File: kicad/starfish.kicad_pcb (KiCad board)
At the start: 2 copper layers, 50 x 38.4 mm, 6 parts, among them J1 Conn_01x09, J2 conn1, J3 Conn_01x08, J4 Conn_01x08, J5 conn2, J6 Conn_01x05

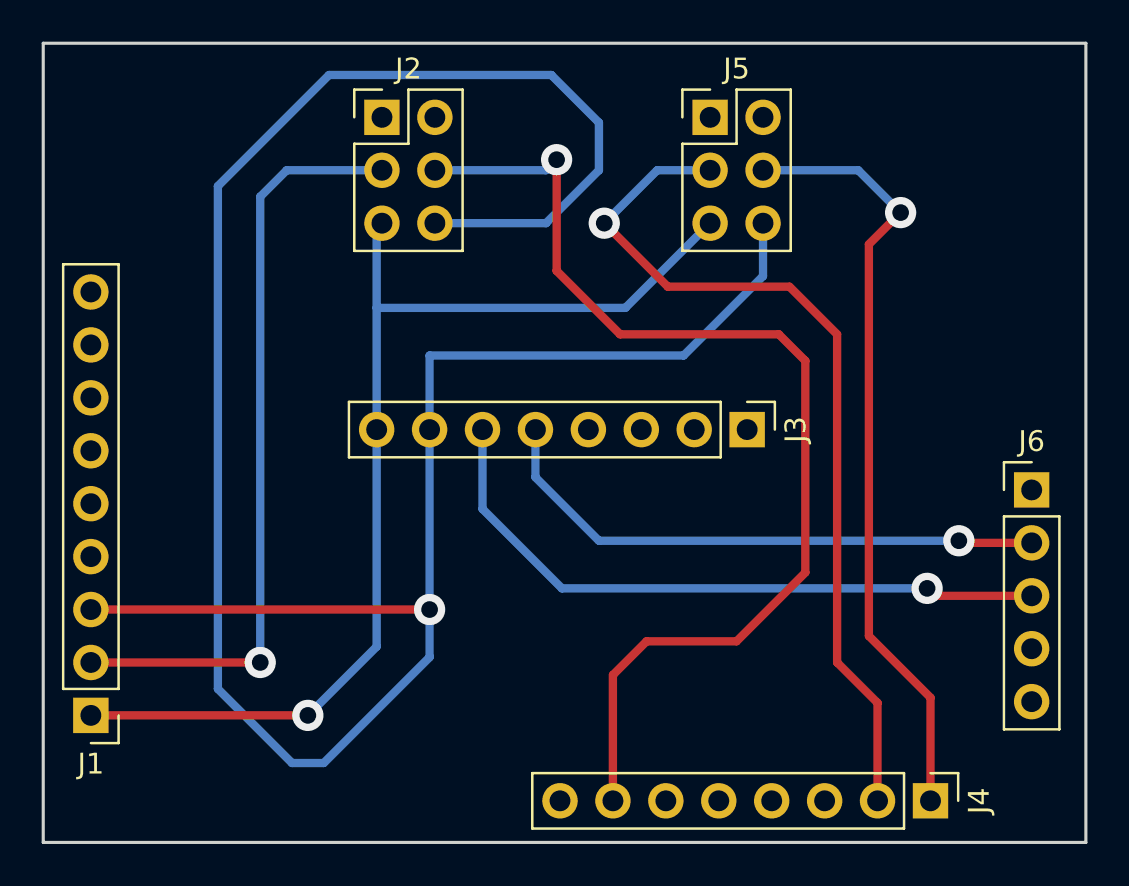
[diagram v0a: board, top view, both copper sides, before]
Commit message: shield
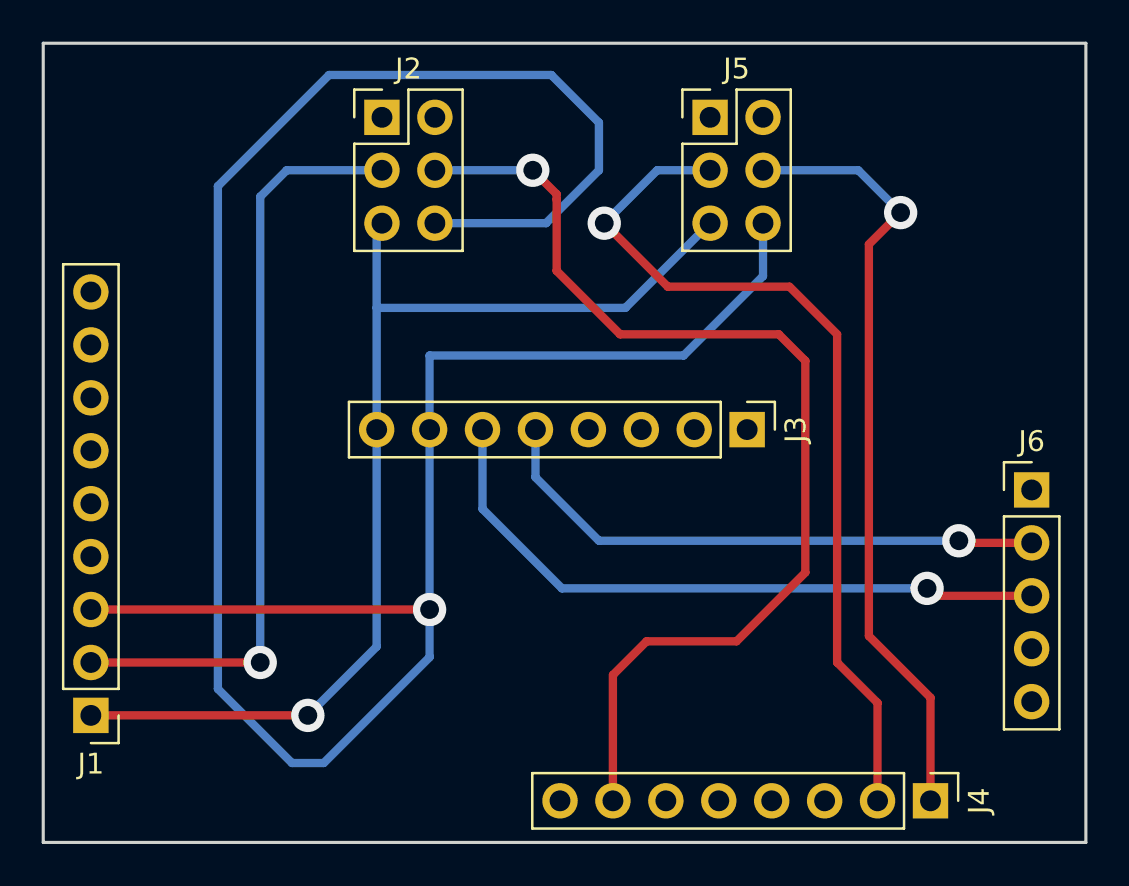
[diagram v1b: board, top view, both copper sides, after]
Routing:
- net Net-(J2-Pad2): track 52.6 -> 51.2 mm
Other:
- net class Default: via_dia 1.5 -> 1.6; via_drill 0.8 -> 0.9
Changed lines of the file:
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@@
     (links 13)
     (no_connects 1)
-    (area 116.510999 104.826999 166.699001 143.331001)
+    (area 116.246999 104.553 166.699001 143.884561)
     (thickness 1.6)
     (drawings 4)
-    (tracks 72)
+    (tracks 74)
     (zones 0)
     (modules 6)
@@
     (segment_width 0.2)
     (edge_width 0.15)
-    (via_size 1.5)
-    (via_drill 0.8)
+    (via_size 1.6)
+    (via_drill 0.9)
     (via_min_size 0.4)
     (via_min_drill 0.3)
@@
     (visible_elements 7FFFFFFF)
     (pcbplotparams
-      (layerselection 0x00000_80000001)
+      (layerselection 0x01000_80000001)
       (usegerberextensions false)
       (excludeedgelayer true)
@@
     (clearance 0.8)
     (trace_width 0.4)
-    (via_dia 1.5)
-    (via_drill 0.8)
+    (via_dia 1.6)
+    (via_drill 0.9)
     (uvia_dia 0.3)
     (uvia_drill 0.1)
@@
   (gr_line (start 166.624 143.256) (end 116.586 143.256) (angle 90) (layer Edge.Cuts) (width 0.15))
   (segment (start 132.588 117.602) (end 144.526 117.602) (width 0.4) (layer B.Cu) (net 1))
-  (segment (start 144.526 117.602) (end 148.59 113.538) (width 0.4) (layer B.Cu) (net 1) (status 800000))
+  (segment (start 144.526 117.602) (end 148.59 113.538) (width 0.4) (layer B.Cu) (net 1))
   (segment (start 132.588 123.444) (end 132.588 117.602) (width 0.4) (layer B.Cu) (net 1))
   (segment (start 132.588 117.602) (end 132.588 113.792) (width 0.4) (layer B.Cu) (net 1))
@@
   (segment (start 132.588 133.858) (end 132.588 123.444) (width 0.4) (layer B.Cu) (net 1))
   (segment (start 129.286 137.16) (end 132.588 133.858) (width 0.4) (layer B.Cu) (net 1))
-  (via (at 129.286 137.16) (size 1.5) (drill 0.8) (layers F.Cu B.Cu) (net 1))
-  (segment (start 132.842 110.998) (end 128.27 110.998) (width 0.4) (layer B.Cu) (net 2) (status 400000))
-  (segment (start 127 134.62) (end 118.872 134.62) (width 0.4) (layer F.Cu) (net 2) (status 800000))
-  (via (at 127 134.62) (size 1.5) (drill 0.8) (layers F.Cu B.Cu) (net 2))
+  (via (at 129.286 137.16) (size 1.6) (drill 0.9) (layers F.Cu B.Cu) (net 1))
+  (segment (start 132.842 110.998) (end 128.27 110.998) (width 0.4) (layer B.Cu) (net 2))
+  (segment (start 127 134.62) (end 118.872 134.62) (width 0.4) (layer F.Cu) (net 2))
+  (via (at 127 134.62) (size 1.6) (drill 0.9) (layers F.Cu B.Cu) (net 2))
   (segment (start 127 112.268) (end 127 134.62) (width 0.4) (layer B.Cu) (net 2))
   (segment (start 128.27 110.998) (end 127 112.268) (width 0.4) (layer B.Cu) (net 2))
   (segment (start 135.128 132.08) (end 135.128 134.366) (width 0.4) (layer B.Cu) (net 3))
-  (segment (start 140.716 113.538) (end 135.382 113.538) (width 0.4) (layer B.Cu) (net 3) (status 800000))
+  (segment (start 140.716 113.538) (end 135.382 113.538) (width 0.4) (layer B.Cu) (net 3))
   (segment (start 143.256 110.998) (end 140.716 113.538) (width 0.4) (layer B.Cu) (net 3))
   (segment (start 143.256 108.712) (end 143.256 110.998) (width 0.4) (layer B.Cu) (net 3))
@@
   (segment (start 130.048 139.446) (end 128.524 139.446) (width 0.4) (layer B.Cu) (net 3))
   (segment (start 135.128 134.366) (end 130.048 139.446) (width 0.4) (layer B.Cu) (net 3))
-  (segment (start 151.13 113.538) (end 151.13 116.078) (width 0.4) (layer B.Cu) (net 3) (status 400000))
+  (segment (start 151.13 113.538) (end 151.13 116.078) (width 0.4) (layer B.Cu) (net 3))
   (segment (start 147.32 119.888) (end 135.128 119.888) (width 0.4) (layer B.Cu) (net 3))
   (segment (start 151.13 116.078) (end 147.32 119.888) (width 0.4) (layer B.Cu) (net 3))
@@
   (segment (start 118.872 132.08) (end 135.128 132.08) (width 0.4) (layer F.Cu) (net 3))
   (segment (start 135.128 132.08) (end 135.128 123.444) (width 0.4) (layer B.Cu) (net 3))
-  (via (at 135.128 132.08) (size 1.5) (drill 0.8) (layers F.Cu B.Cu) (net 3))
-  (segment (start 164.02304 128.8796) (end 160.6296 128.8796) (width 0.4) (layer F.Cu) (net 16) (status 400000))
-  (segment (start 140.208 125.73) (end 140.208 123.444) (width 0.4) (layer B.Cu) (net 16) (status 800000))
+  (via (at 135.128 132.08) (size 1.6) (drill 0.9) (layers F.Cu B.Cu) (net 3))
+  (segment (start 164.02304 128.8796) (end 160.6296 128.8796) (width 0.4) (layer F.Cu) (net 16))
+  (segment (start 140.208 125.73) (end 140.208 123.444) (width 0.4) (layer B.Cu) (net 16))
   (segment (start 143.256 128.778) (end 140.208 125.73) (width 0.4) (layer B.Cu) (net 16))
   (segment (start 160.528 128.778) (end 143.256 128.778) (width 0.4) (layer B.Cu) (net 16))
-  (via (at 160.528 128.778) (size 1.5) (drill 0.8) (layers F.Cu B.Cu) (net 16))
+  (via (at 160.528 128.778) (size 1.6) (drill 0.9) (layers F.Cu B.Cu) (net 16))
   (segment (start 160.6296 128.8796) (end 160.528 128.778) (width 0.4) (layer F.Cu) (net 16))
-  (segment (start 164.02304 131.4196) (end 159.3596 131.4196) (width 0.4) (layer F.Cu) (net 17) (status 400000))
-  (segment (start 137.668 127.254) (end 137.668 123.444) (width 0.4) (layer B.Cu) (net 17) (status 800000))
+  (segment (start 164.02304 131.4196) (end 159.3596 131.4196) (width 0.4) (layer F.Cu) (net 17))
+  (segment (start 137.668 127.254) (end 137.668 123.444) (width 0.4) (layer B.Cu) (net 17))
   (segment (start 141.478 131.064) (end 137.668 127.254) (width 0.4) (layer B.Cu) (net 17))
   (segment (start 159.004 131.064) (end 141.478 131.064) (width 0.4) (layer B.Cu) (net 17))
-  (via (at 159.004 131.064) (size 1.5) (drill 0.8) (layers F.Cu B.Cu) (net 17))
+  (via (at 159.004 131.064) (size 1.6) (drill 0.9) (layers F.Cu B.Cu) (net 17))
   (segment (start 159.3596 131.4196) (end 159.004 131.064) (width 0.4) (layer F.Cu) (net 17))
-  (segment (start 148.59 110.998) (end 146.05 110.998) (width 0.4) (layer B.Cu) (net 18) (status 400000))
-  (segment (start 156.62656 136.56056) (end 156.62656 141.25956) (width 0.4) (layer F.Cu) (net 18) (status 800000))
+  (segment (start 148.59 110.998) (end 146.05 110.998) (width 0.4) (layer B.Cu) (net 18))
+  (segment (start 156.62656 136.56056) (end 156.62656 141.25956) (width 0.4) (layer F.Cu) (net 18))
   (segment (start 154.686 134.62) (end 156.62656 136.56056) (width 0.4) (layer F.Cu) (net 18))
   (segment (start 154.686 118.872) (end 154.686 134.62) (width 0.4) (layer F.Cu) (net 18))
@@
   (segment (start 146.558 116.586) (end 152.4 116.586) (width 0.4) (layer F.Cu) (net 18))
   (segment (start 143.51 113.538) (end 146.558 116.586) (width 0.4) (layer F.Cu) (net 18))
-  (via (at 143.51 113.538) (size 1.5) (drill 0.8) (layers F.Cu B.Cu) (net 18))
+  (via (at 143.51 113.538) (size 1.6) (drill 0.9) (layers F.Cu B.Cu) (net 18))
   (segment (start 146.05 110.998) (end 143.51 113.538) (width 0.4) (layer B.Cu) (net 18))
-  (segment (start 135.382 110.998) (end 140.716 110.998) (width 0.4) (layer B.Cu) (net 27) (status 400000))
-  (segment (start 143.92656 135.21944) (end 143.92656 141.25956) (width 0.4) (layer F.Cu) (net 27) (status 800000))
+  (segment (start 139.7 110.998) (end 140.081 110.998) (width 0.4) (layer B.Cu) (net 27))
+  (segment (start 141.224 112.395) (end 141.224 115.824) (width 0.4) (layer F.Cu) (net 27))
+  (segment (start 141.224 115.824) (end 144.272 118.872) (width 0.4) (layer F.Cu) (net 27))
+  (segment (start 144.272 118.872) (end 151.892 118.872) (width 0.4) (layer F.Cu) (net 27))
+  (segment (start 151.892 118.872) (end 153.162 120.142) (width 0.4) (layer F.Cu) (net 27))
+  (segment (start 153.162 120.142) (end 153.162 130.302) (width 0.4) (layer F.Cu) (net 27))
+  (segment (start 153.162 130.302) (end 149.86 133.604) (width 0.4) (layer F.Cu) (net 27))
+  (segment (start 149.86 133.604) (end 145.542 133.604) (width 0.4) (layer F.Cu) (net 27))
   (segment (start 145.542 133.604) (end 143.92656 135.21944) (width 0.4) (layer F.Cu) (net 27))
-  (segment (start 149.86 133.604) (end 145.542 133.604) (width 0.4) (layer F.Cu) (net 27))
-  (segment (start 153.162 130.302) (end 149.86 133.604) (width 0.4) (layer F.Cu) (net 27))
-  (segment (start 153.162 120.142) (end 153.162 130.302) (width 0.4) (layer F.Cu) (net 27))
-  (segment (start 151.892 118.872) (end 153.162 120.142) (width 0.4) (layer F.Cu) (net 27))
-  (segment (start 144.272 118.872) (end 151.892 118.872) (width 0.4) (layer F.Cu) (net 27))
-  (segment (start 141.224 115.824) (end 144.272 118.872) (width 0.4) (layer F.Cu) (net 27))
-  (segment (start 141.224 110.49) (end 141.224 115.824) (width 0.4) (layer F.Cu) (net 27))
-  (via (at 141.224 110.49) (size 1.5) (drill 0.8) (layers F.Cu B.Cu) (net 27))
-  (segment (start 140.716 110.998) (end 141.224 110.49) (width 0.4) (layer B.Cu) (net 27))
-  (segment (start 151.13 110.998) (end 155.702 110.998) (width 0.4) (layer B.Cu) (net 28) (status 400000))
-  (segment (start 159.16656 136.30656) (end 159.16656 141.25956) (width 0.4) (layer F.Cu) (net 28) (status 800000))
+  (segment (start 143.92656 141.25956) (end 143.92656 135.21944) (width 0.4) (layer F.Cu) (net 27))
+  (segment (start 139.7 110.998) (end 135.382 110.998) (width 0.4) (layer B.Cu) (net 27) (status 800000))
+  (segment (start 141.224 112.141) (end 141.224 112.395) (width 0.4) (layer F.Cu) (net 27))
+  (segment (start 140.081 110.998) (end 141.224 112.141) (width 0.4) (layer F.Cu) (net 27))
+  (via (at 140.081 110.998) (size 1.6) (drill 0.9) (layers F.Cu B.Cu) (net 27))
+  (segment (start 151.13 110.998) (end 155.702 110.998) (width 0.4) (layer B.Cu) (net 28))
+  (segment (start 159.16656 136.30656) (end 159.16656 141.25956) (width 0.4) (layer F.Cu) (net 28))
   (segment (start 156.21 133.35) (end 159.16656 136.30656) (width 0.4) (layer F.Cu) (net 28))
   (segment (start 156.21 114.554) (end 156.21 133.35) (width 0.4) (layer F.Cu) (net 28))
   (segment (start 157.734 113.03) (end 156.21 114.554) (width 0.4) (layer F.Cu) (net 28))
-  (via (at 157.734 113.03) (size 1.5) (drill 0.8) (layers F.Cu B.Cu) (net 28))
+  (via (at 157.734 113.03) (size 1.6) (drill 0.9) (layers F.Cu B.Cu) (net 28))
   (segment (start 155.702 110.998) (end 157.734 113.03) (width 0.4) (layer B.Cu) (net 28))
 )
